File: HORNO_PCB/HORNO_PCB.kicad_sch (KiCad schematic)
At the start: 105 parts, among them J0_1 Terminales de tornillo espaci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, J0_10 Terminales de tornillo espaci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, J0_13 Terminales de tornillo espaci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, J0_14 Terminales de tornillo espaci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, J0_18 Terminales de tornillo espaci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, J0_3 Terminales de tornillo espaci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, J0_4 Terminales de tornillo espaci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, J0_5 Terminales de tornillo espaci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, J0_6 Terminales de tornillo espaci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, J0_7 Terminales de tornillo espaci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, J0_8 Terminales de tornillo espaci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, J0_9 Terminales de tornillo espaci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, J1 switch, J10 switch, J11 switch, J12 switch, J13 switch, J14 switch, J15 switch, J16 switch, J17 switch, J18 switch, J19 switch, J2 switch, J20 switch, J21 switch, J22 switch, J23 switch, J24 Screw_Terminal_01x20, J25 Screw_Terminal_01x20, J26 Screw_Terminal_01x20, J27 Screw_Terminal_01x20, J3 switch, J4 switch, J5 switch, J6 switch, J7 24VDC, J8 switch, J9 switch, K1 Relay 1, K2 Relay 2, K6 Relay 4, K7 Relay 3, K8 Relay 2, K9 Relay 1, Q1 2N2222, Q2 2N2222, Q6 IRG4PF50W, Q7 IRG4PF50W, U1 TLP521-1, U10 LM741, U15 TLP250, U17 LM741, U18 LM741, U19 TLP250, U2 TLP521-1, U25 UDN2981A, U3 TLP521-1, U4 TLP521-1, U9 LM741

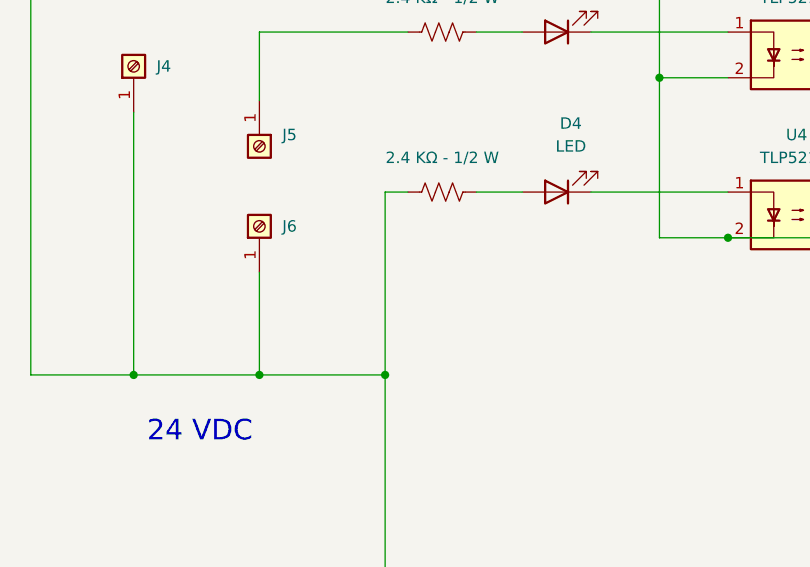
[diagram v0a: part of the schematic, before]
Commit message: Actualización de PCB
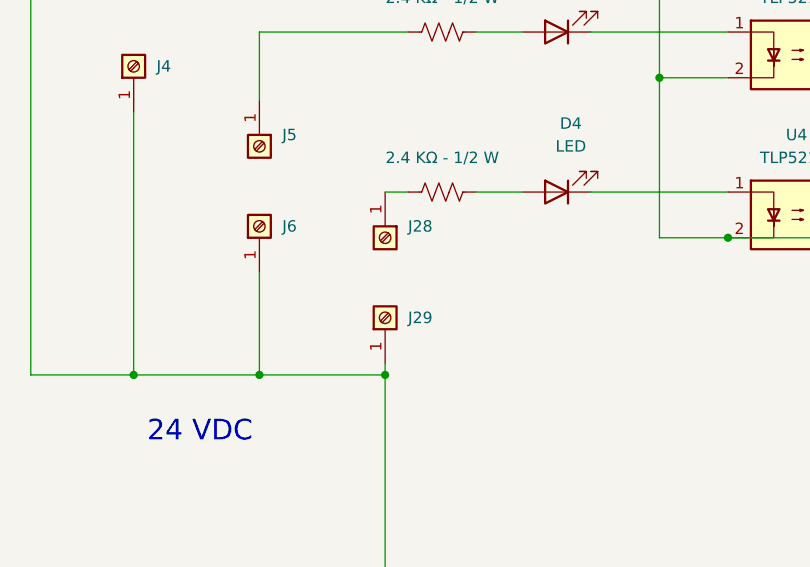
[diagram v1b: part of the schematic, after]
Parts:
- added J28, J29: switch, TerminalBlock_MetzConnect:TerminalBlock_MetzConnect_360271_1x01_Horizontal_ScrewM3.0_Boxed, symbol Connector:Screw_Terminal_01x01
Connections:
- net at D10.2 (A), D11.2 (A), D12.2 (A)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: now also J29.1 (Pin_1); no longer R12.1
- new net: J28.1 (Pin_1), R12.1
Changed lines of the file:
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@@
 	)
 	(junction
-		(at 133.35 353.06)
-		(diameter 0)
-		(color 0 0 0 0)
-	)
-	(junction
 		(at 568.96 273.05)
 		(diameter 0)
@@
 	)
 	(junction
+		(at 105.41 353.06)
+		(diameter 0)
+		(color 0 0 0 0)
+	)
+	(junction
 		(at 839.47 570.23)
 		(diameter 0)
@@
 	)
 	(junction
+		(at 119.38 353.06)
+		(diameter 0)
+		(color 0 0 0 0)
+	)
+	(junction
 		(at 212.09 314.96)
 		(diameter 0)
@@
 	)
 	(junction
-		(at 119.38 353.06)
-		(diameter 0)
-		(color 0 0 0 0)
-	)
-	(junction
 		(at 1112.52 373.38)
 		(diameter 0)
@@
 	)
 	(junction
-		(at 105.41 353.06)
+		(at 683.26 462.28)
 		(diameter 0)
 		(color 0 0 0 0)
 	)
 	(junction
-		(at 683.26 462.28)
+		(at 918.21 482.6)
 		(diameter 0)
 		(color 0 0 0 0)
 	)
 	(junction
-		(at 918.21 482.6)
+		(at 186.69 337.82)
 		(diameter 0)
 		(color 0 0 0 0)
 	)
 	(junction
-		(at 186.69 337.82)
+		(at 133.35 353.06)
 		(diameter 0)
 		(color 0 0 0 0)
@@
 	(wire
 		(pts
-			(xy 105.41 353.06) (xy 119.38 353.06)
-		)
-		(stroke
-			(width 0)
-			(type default)
-			(color 255 11 0 1)
-		)
-	)
-	(wire
-		(pts
 			(xy 278.13 200.66) (xy 278.13 289.56)
 		)
@@
 	(wire
 		(pts
-			(xy 119.38 353.06) (xy 133.35 353.06)
-		)
-		(stroke
-			(width 0)
-			(type default)
-			(color 255 11 0 1)
-		)
-	)
-	(wire
-		(pts
 			(xy 466.09 147.32) (xy 513.08 147.32)
 		)
@@
 	(wire
 		(pts
+			(xy 133.35 351.79) (xy 133.35 353.06)
+		)
+		(stroke
+			(width 0)
+			(type default)
+			(color 255 11 0 1)
+		)
+	)
+	(wire
+		(pts
 			(xy 133.35 772.16) (xy 632.46 772.16)
 		)
@@
 	(wire
 		(pts
+			(xy 93.98 353.06) (xy 105.41 353.06)
+		)
+		(stroke
+			(width 0)
+			(type default)
+			(color 255 11 0 1)
+		)
+	)
+	(wire
+		(pts
 			(xy 431.8 554.99) (xy 431.8 541.02)
 		)
@@
 	(wire
 		(pts
-			(xy 93.98 353.06) (xy 105.41 353.06)
-		)
-		(stroke
-			(width 0)
-			(type default)
-			(color 255 11 0 1)
-		)
-	)
-	(wire
-		(pts
-			(xy 133.35 332.74) (xy 133.35 353.06)
-		)
-		(stroke
-			(width 0)
-			(type default)
-			(color 255 11 0 1)
-		)
-	)
-	(wire
-		(pts
 			(xy 872.49 549.91) (xy 872.49 582.93)
 		)
@@
 	(wire
 		(pts
-			(xy 133.35 353.06) (xy 133.35 772.16)
-		)
-		(stroke
-			(width 0)
-			(type default)
-			(color 255 11 0 1)
-		)
-	)
-	(wire
-		(pts
 			(xy 436.88 629.92) (xy 436.88 562.61)
 		)
@@
 	(wire
 		(pts
+			(xy 119.38 353.06) (xy 133.35 353.06)
+		)
+		(stroke
+			(width 0)
+			(type default)
+			(color 255 11 0 1)
+		)
+	)
+	(wire
+		(pts
 			(xy 500.38 622.3) (xy 516.89 622.3)
 		)
@@
 	(wire
 		(pts
+			(xy 105.41 353.06) (xy 119.38 353.06)
+		)
+		(stroke
+			(width 0)
+			(type default)
+			(color 255 11 0 1)
+		)
+	)
+	(wire
+		(pts
 			(xy 383.54 567.69) (xy 387.35 567.69)
 		)
@@
 	(wire
 		(pts
+			(xy 133.35 353.06) (xy 133.35 772.16)
+		)
+		(stroke
+			(width 0)
+			(type default)
+			(color 255 11 0 1)
+		)
+	)
+	(wire
+		(pts
 			(xy 858.52 549.91) (xy 872.49 549.91)
 		)
@@
 	(symbol
 		(lib_id "Connector:Screw_Terminal_01x01")
+		(at 133.35 346.71 90)
+		(unit 1)
+		(exclude_from_sim no)
+		(in_bom yes)
+		(on_board yes)
+		(dnp no)
+		(fields_autoplaced yes)
+		(property "Reference" "J29"
+			(at 135.89 346.7099 90)
+			(effects
+				(font
+					(size 1.27 1.27)
+				)
+				(justify right)
+			)
+		)
+		(property "Value" "switch"
+			(at 130.81 345.4401 90)
+			(effects
+				(font
+					(size 1.27 1.27)
+				)
+				(justify left)
+				(hide yes)
+			)
+		)
+		(property "Footprint" "TerminalBlock_MetzConnect:TerminalBlock_MetzConnect_360271_1x01_Horizontal_ScrewM3.0_Boxed"
+			(at 133.35 346.71 0)
+			(effects
+				(font
+					(size 1.27 1.27)
+				)
+				(hide yes)
+			)
+		)
+		(property "Datasheet" "~"
+			(at 133.35 346.71 0)
+			(effects
+				(font
+					(size 1.27 1.27)
+				)
+				(hide yes)
+			)
+		)
+		(property "Description" "Generic screw terminal, single row, 01x01, script generated (kicad-library-utils/schlib/autogen/connector/)"
+			(at 133.35 346.71 0)
+			(effects
+				(font
+					(size 1.27 1.27)
+				)
+				(hide yes)
+			)
+		)
+		(pin "1"
+		)
+		(instances
+			(project "HORNO_PCB"
+				(path "/70384b34-09dd-4fe3-975b-9645e85de3d4"
+					(reference "J29")
+					(unit 1)
+				)
+			)
+		)
+	)
+	(symbol
+		(lib_id "Connector:Screw_Terminal_01x01")
 		(at 684.53 662.94 90)
 		(unit 1)
@@
 					(unit 1)
 				)
+			)
+		)
+	)
+	(symbol
+		(lib_id "Connector:Screw_Terminal_01x01")
+		(at 133.35 337.82 270)
+		(unit 1)
+		(exclude_from_sim no)
+		(in_bom yes)
+		(on_board yes)
+		(dnp no)
+		(fields_autoplaced yes)
+		(property "Reference" "J28"
+			(at 135.89 336.5499 90)
+			(effects
+				(font
+					(size 1.27 1.27)
+				)
+				(justify left)
+			)
+		)
+		(property "Value" "switch"
+			(at 135.89 339.0899 90)
+			(effects
+				(font
+					(size 1.27 1.27)
+				)
+				(justify left)
+				(hide yes)
+			)
+		)
+		(property "Footprint" "TerminalBlock_MetzConnect:TerminalBlock_MetzConnect_360271_1x01_Horizontal_ScrewM3.0_Boxed"
+			(at 133.35 337.82 0)
+			(effects
+				(font
+					(size 1.27 1.27)
+				)
+				(hide yes)
+			)
+		)
+		(property "Datasheet" "~"
+			(at 133.35 337.82 0)
+			(effects
+				(font
+					(size 1.27 1.27)
+				)
+				(hide yes)
+			)
+		)
+		(property "Description" "Generic screw terminal, single row, 01x01, script generated (kicad-library-utils/schlib/autogen/connector/)"
+			(at 133.35 337.82 0)
+			(effects
+				(font
+					(size 1.27 1.27)
+				)
+				(hide yes)
+			)
+		)
+		(pin "1"
+		)
+		(instances
+			(project "HORNO_PCB"
+				(path "/70384b34-09dd-4fe3-975b-9645e85de3d4"
+					(reference "J28")
+					(unit 1)
+				)

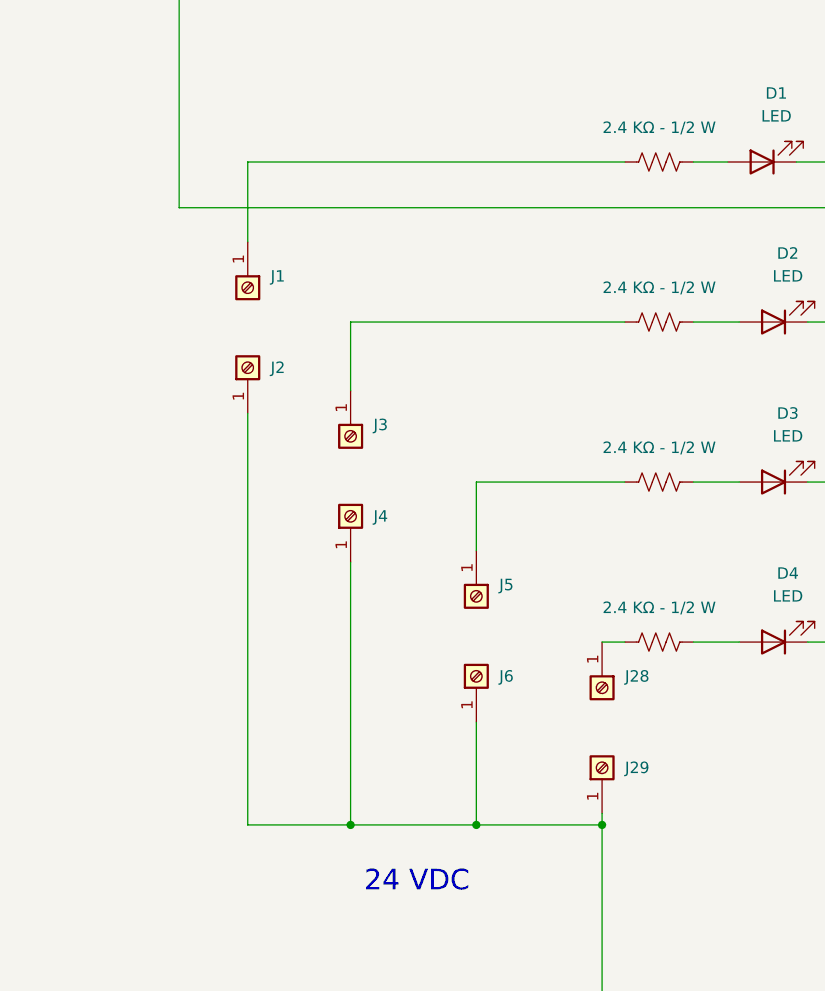
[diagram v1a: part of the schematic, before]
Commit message: Actualizacion de PCB
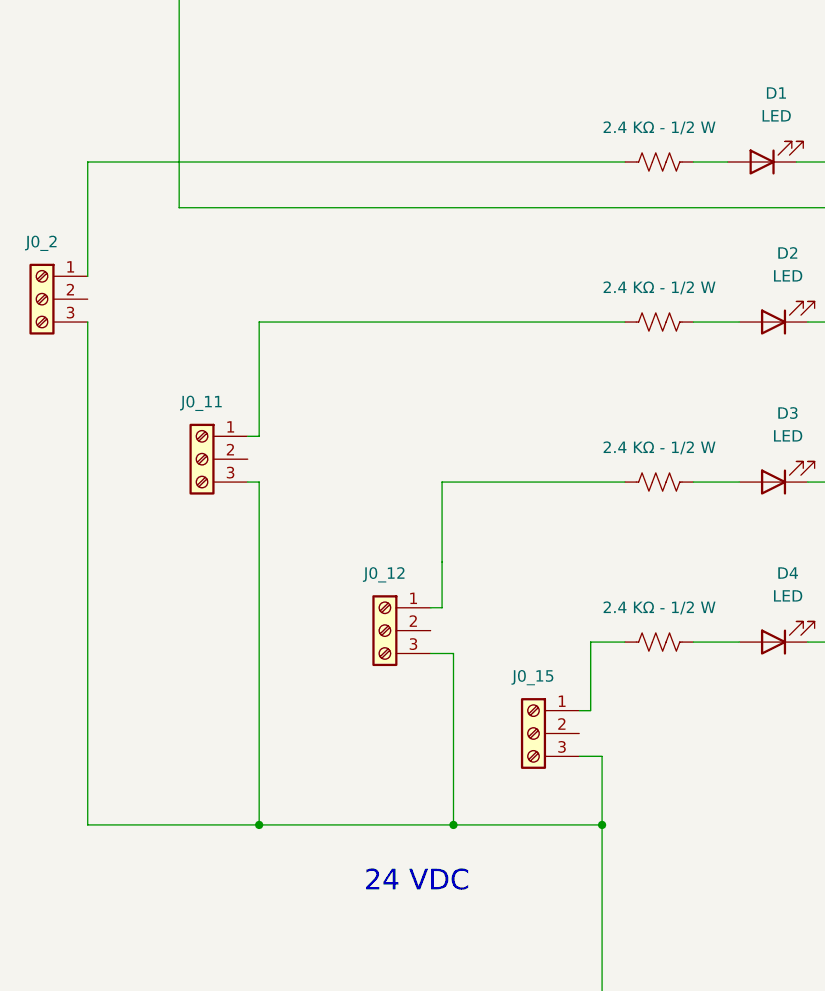
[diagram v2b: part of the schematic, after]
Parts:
- removed J1, J2, J28, J29, J3, J4, J5, J6: switch, TerminalBlock_MetzConnect:TerminalBlock_MetzConnect_360271_1x01_Horizontal_ScrewM3.0_Boxed, symbol Connector:Screw_Terminal_01x01
- added J0_11, J0_12, J0_15, J0_2: Terminales de tornillo espaciados en 5mm, TerminalBlock_Phoenix:TerminalBlock_Phoenix_PT-1,5-3-5.0-H_1x03_P5.00mm_Horizontal, symbol Connector:Screw_Terminal_01x03
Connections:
- net at R7.1: now also J0_11.1 (Pin_1)
- net at D10.2 (A), D11.2 (A), D12.2 (A)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: now also J0_11.3 (Pin_3), J0_12.3 (Pin_3), J0_15.3 (Pin_3), J0_2.3 (Pin_3)
- net at R8.1: now also J0_12.1 (Pin_1)
- net at R28.1: now also J0_2.1 (Pin_1)
- net at R12.1: now also J0_15.1 (Pin_1)

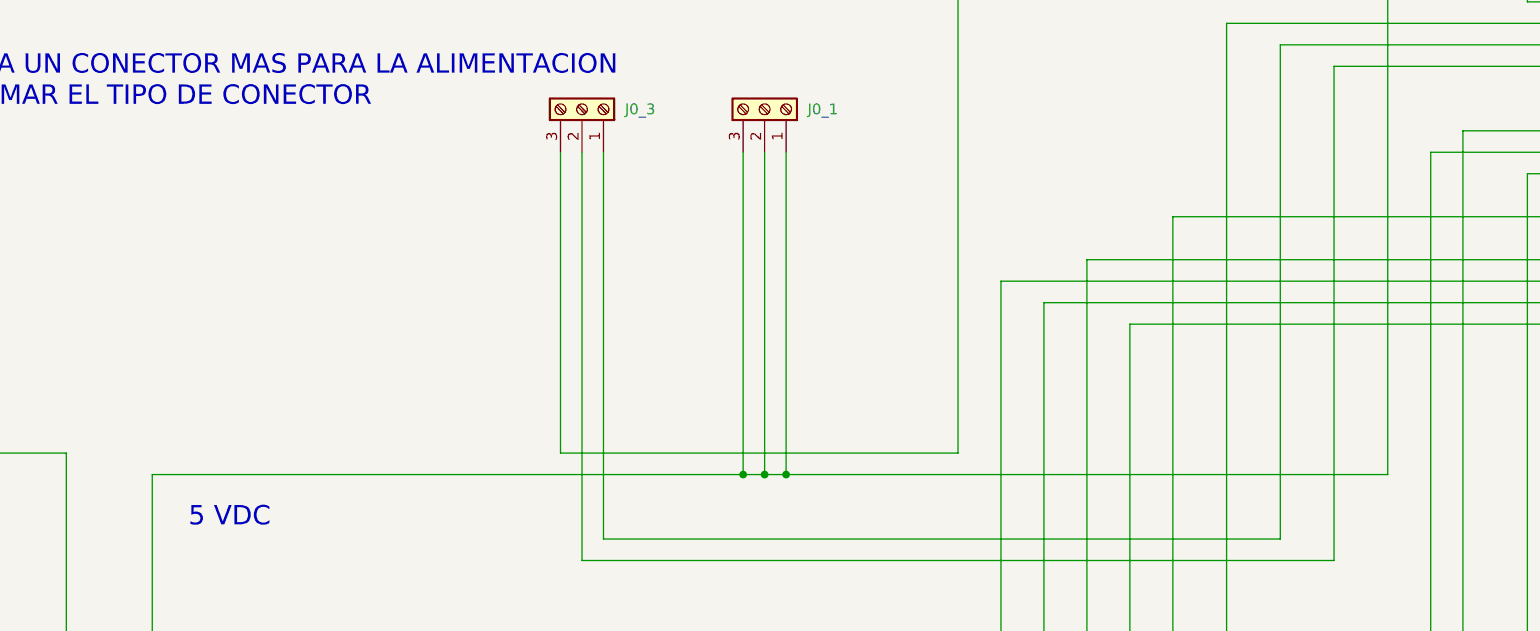
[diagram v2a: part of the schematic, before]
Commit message: Actualizacion de PCB
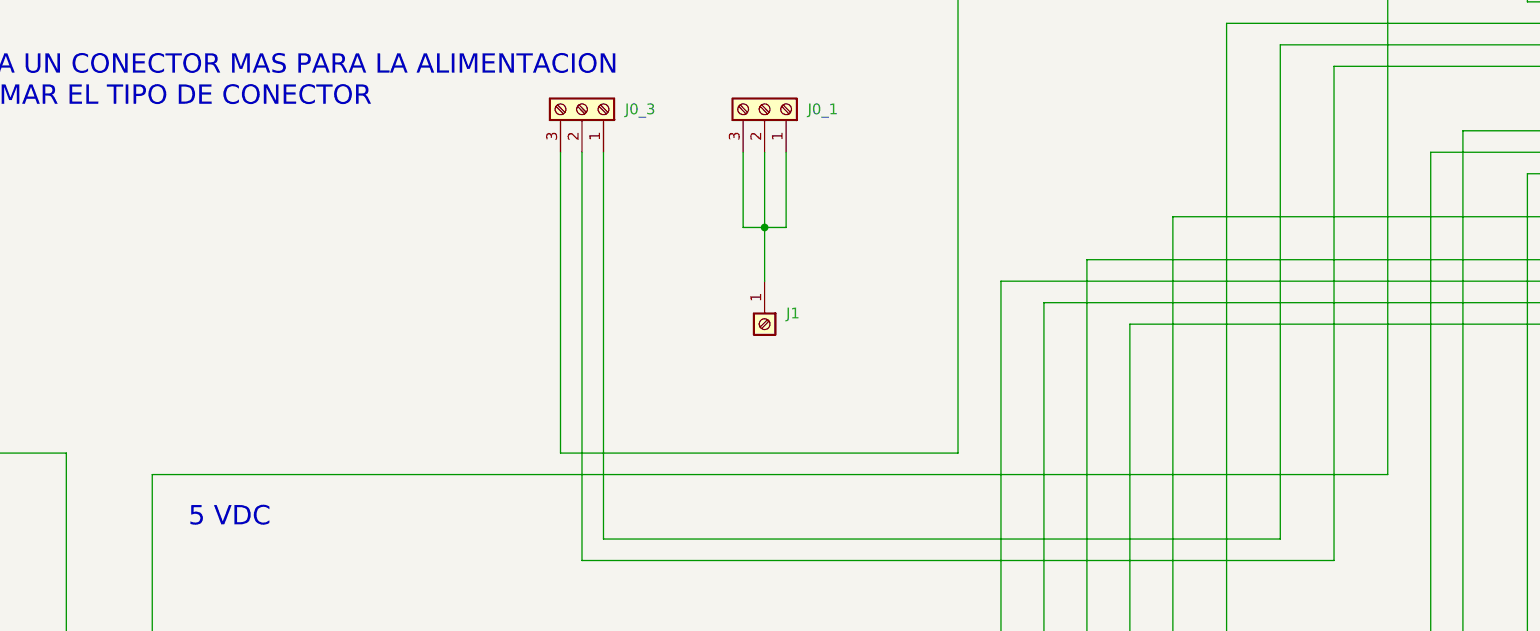
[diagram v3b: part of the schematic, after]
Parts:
- added J1: switch, TerminalBlock_MetzConnect:TerminalBlock_MetzConnect_360271_1x01_Horizontal_ScrewM3.0_Boxed, symbol Connector:Screw_Terminal_01x01
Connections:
- net at J11.1 (Pin_1), J21.1 (Pin_1), J24.2 (Pin_2)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: no longer J0_1.1 (Pin_1), J0_1.2 (Pin_2), J0_1.3 (Pin_3)
- new net: J0_1.1 (Pin_1), J0_1.2 (Pin_2), J0_1.3 (Pin_3), J1.1 (Pin_1)
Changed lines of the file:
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@@
 	)
 	(junction
-		(at 492.76 149.86)
-		(diameter 0)
-		(color 0 0 0 0)
-	)
-	(junction
 		(at 622.3 675.64)
 		(diameter 0)
@@
 	)
 	(junction
-		(at 487.68 149.86)
-		(diameter 0)
-		(color 0 0 0 0)
-	)
-	(junction
 		(at 977.9 336.55)
 		(diameter 0)
@@
 	)
 	(junction
-		(at 490.22 149.86)
+		(at 490.22 120.65)
 		(diameter 0)
 		(color 0 0 0 0)
@@
 	(wire
 		(pts
+			(xy 490.22 111.76) (xy 490.22 120.65)
+		)
+		(stroke
+			(width 0)
+			(type default)
+			(color 255 6 0 1)
+		)
+	)
+	(wire
+		(pts
 			(xy 825.5 120.65) (xy 652.78 120.65)
 		)
@@
 	(wire
 		(pts
-			(xy 490.22 149.86) (xy 492.76 149.86)
+			(xy 191.77 314.96) (xy 195.58 314.96)
 		)
 		(stroke
 			(width 0)
 			(type default)
-			(color 255 6 0 1)
 		)
 	)
 	(wire
 		(pts
-			(xy 191.77 314.96) (xy 195.58 314.96)
+			(xy 763.27 462.28) (xy 763.27 525.78)
 		)
 		(stroke
@@
 	(wire
 		(pts
-			(xy 763.27 462.28) (xy 763.27 525.78)
+			(xy 464.82 629.92) (xy 478.79 629.92)
 		)
 		(stroke
@@
 	(wire
 		(pts
-			(xy 464.82 629.92) (xy 478.79 629.92)
+			(xy 417.83 622.3) (xy 433.07 622.3)
 		)
 		(stroke
@@
 	(wire
 		(pts
-			(xy 417.83 622.3) (xy 433.07 622.3)
+			(xy 887.73 486.41) (xy 887.73 603.25)
 		)
 		(stroke
 			(width 0)
 			(type default)
+			(color 0 0 0 1)
 		)
 	)
 	(wire
 		(pts
-			(xy 887.73 486.41) (xy 887.73 603.25)
+			(xy 528.32 170.18) (xy 528.32 124.46)
 		)
 		(stroke
 			(width 0)
 			(type default)
-			(color 0 0 0 1)
 		)
 	)
 	(wire
 		(pts
-			(xy 528.32 170.18) (xy 528.32 124.46)
+			(xy 492.76 111.76) (xy 492.76 120.65)
 		)
 		(stroke
 			(width 0)
 			(type default)
+			(color 255 6 0 1)
 		)
 	)
@@
 	(wire
 		(pts
-			(xy 490.22 111.76) (xy 490.22 149.86)
-		)
-		(stroke
-			(width 0)
-			(type default)
-			(color 255 6 0 1)
-		)
-	)
-	(wire
-		(pts
 			(xy 391.16 629.92) (xy 391.16 562.61)
 		)
@@
 	(wire
 		(pts
+			(xy 490.22 120.65) (xy 490.22 127)
+		)
+		(stroke
+			(width 0)
+			(type default)
+			(color 255 6 0 1)
+		)
+	)
+	(wire
+		(pts
 			(xy 575.31 293.37) (xy 575.31 320.04)
 		)
@@
 	(wire
 		(pts
+			(xy 492.76 120.65) (xy 490.22 120.65)
+		)
+		(stroke
+			(width 0)
+			(type default)
+			(color 255 6 0 1)
+		)
+	)
+	(wire
+		(pts
 			(xy 674.37 477.52) (xy 665.48 477.52)
 		)
@@
 	(wire
 		(pts
-			(xy 417.83 149.86) (xy 487.68 149.86)
-		)
-		(stroke
-			(width 0)
-			(type default)
-			(color 255 6 0 1)
-		)
-	)
-	(wire
-		(pts
 			(xy 822.96 666.75) (xy 822.96 683.26)
 		)
@@
 	(wire
 		(pts
-			(xy 487.68 111.76) (xy 487.68 149.86)
-		)
-		(stroke
-			(width 0)
-			(type default)
-			(color 255 6 0 1)
-		)
-	)
-	(wire
-		(pts
 			(xy 481.33 463.55) (xy 496.57 463.55)
 		)
@@
 	(wire
 		(pts
-			(xy 492.76 149.86) (xy 563.88 149.86)
+			(xy 417.83 149.86) (xy 563.88 149.86)
 		)
 		(stroke
@@
 	(wire
 		(pts
+			(xy 487.68 111.76) (xy 487.68 120.65)
+		)
+		(stroke
+			(width 0)
+			(type default)
+			(color 255 6 0 1)
+		)
+	)
+	(wire
+		(pts
 			(xy 593.09 116.84) (xy 588.01 116.84)
 		)
@@
 	(wire
 		(pts
-			(xy 492.76 111.76) (xy 492.76 149.86)
-		)
-		(stroke
-			(width 0)
-			(type default)
-			(color 255 6 0 1)
-		)
-	)
-	(wire
-		(pts
 			(xy 171.45 284.48) (xy 163.83 284.48)
 		)
@@
 	(wire
 		(pts
-			(xy 695.96 110.49) (xy 652.78 110.49)
+			(xy 487.68 120.65) (xy 490.22 120.65)
 		)
 		(stroke
 			(width 0)
 			(type default)
+			(color 255 6 0 1)
 		)
 	)
 	(wire
 		(pts
-			(xy 669.29 441.96) (xy 669.29 440.69)
+			(xy 695.96 110.49) (xy 652.78 110.49)
 		)
 		(stroke
 			(width 0)
 			(type default)
-			(color 0 0 0 1)
 		)
 	)
 	(wire
 		(pts
-			(xy 789.94 683.26) (xy 789.94 626.11)
+			(xy 669.29 441.96) (xy 669.29 440.69)
 		)
 		(stroke
 			(width 0)
 			(type default)
-			(color 255 6 0 1)
+			(color 0 0 0 1)
 		)
 	)
 	(wire
 		(pts
-			(xy 505.46 629.92) (xy 520.7 629.92)
+			(xy 789.94 683.26) (xy 789.94 626.11)
 		)
 		(stroke
 			(width 0)
 			(type default)
+			(color 255 6 0 1)
 		)
 	)
 	(wire
 		(pts
-			(xy 487.68 149.86) (xy 490.22 149.86)
+			(xy 505.46 629.92) (xy 520.7 629.92)
 		)
 		(stroke
 			(width 0)
 			(type default)
-			(color 255 6 0 1)
 		)
 	)
@@
 					(unit 1)
 				)
+			)
+		)
+	)
+	(symbol
+		(lib_id "Connector:Screw_Terminal_01x01")
+		(at 490.22 132.08 270)
+		(unit 1)
+		(exclude_from_sim no)
+		(in_bom yes)
+		(on_board yes)
+		(dnp no)
+		(fields_autoplaced yes)
+		(property "Reference" "J1"
+			(at 492.76 130.8099 90)
+			(effects
+				(font
+					(size 1.27 1.27)
+				)
+				(justify left)
+			)
+		)
+		(property "Value" "switch"
+			(at 492.76 133.3499 90)
+			(effects
+				(font
+					(size 1.27 1.27)
+				)
+				(justify left)
+				(hide yes)
+			)
+		)
+		(property "Footprint" "TerminalBlock_MetzConnect:TerminalBlock_MetzConnect_360271_1x01_Horizontal_ScrewM3.0_Boxed"
+			(at 490.22 132.08 0)
+			(effects
+				(font
+					(size 1.27 1.27)
+				)
+				(hide yes)
+			)
+		)
+		(property "Datasheet" "~"
+			(at 490.22 132.08 0)
+			(effects
+				(font
+					(size 1.27 1.27)
+				)
+				(hide yes)
+			)
+		)
+		(property "Description" "Generic screw terminal, single row, 01x01, script generated (kicad-library-utils/schlib/autogen/connector/)"
+			(at 490.22 132.08 0)
+			(effects
+				(font
+					(size 1.27 1.27)
+				)
+				(hide yes)
+			)
+		)
+		(pin "1"
+		)
+		(instances
+			(project "HORNO_PCB"
+				(path "/70384b34-09dd-4fe3-975b-9645e85de3d4"
+					(reference "J1")
+					(unit 1)
+				)
